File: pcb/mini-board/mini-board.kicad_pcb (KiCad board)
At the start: 4 copper layers, 132.1 x 132.1 mm, 55 parts, among them J1 USB_B, J2 EXPANSION BUS, J3 SD Card Board, J4 Atmel-JTAG-10, J5 SYSTEM BUS, J8 SERIAL, SW1 SW_SPDT, SW2 RESET, SW3 NMI, U1 74AC11, U11 DS1813, U15 SST39SF040, U16 AS6C4008-55, U19 W65C22S, U2 W65C02, U21 W65C51N, U22 MAX232, U23 ATF1502AS, X1 CLK, Y1 1.8432 MHz

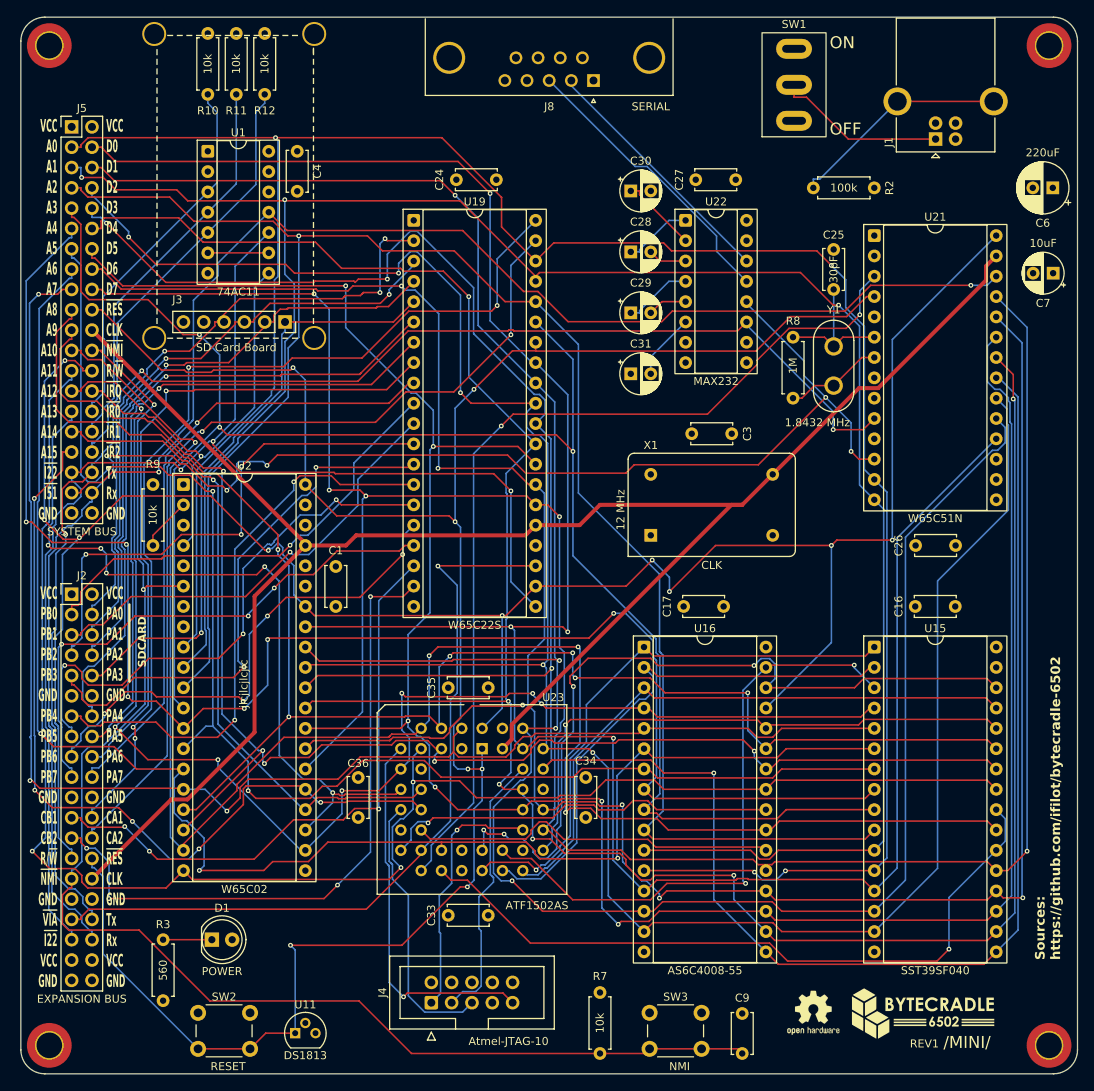
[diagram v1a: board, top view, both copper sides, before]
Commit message: Rivising board
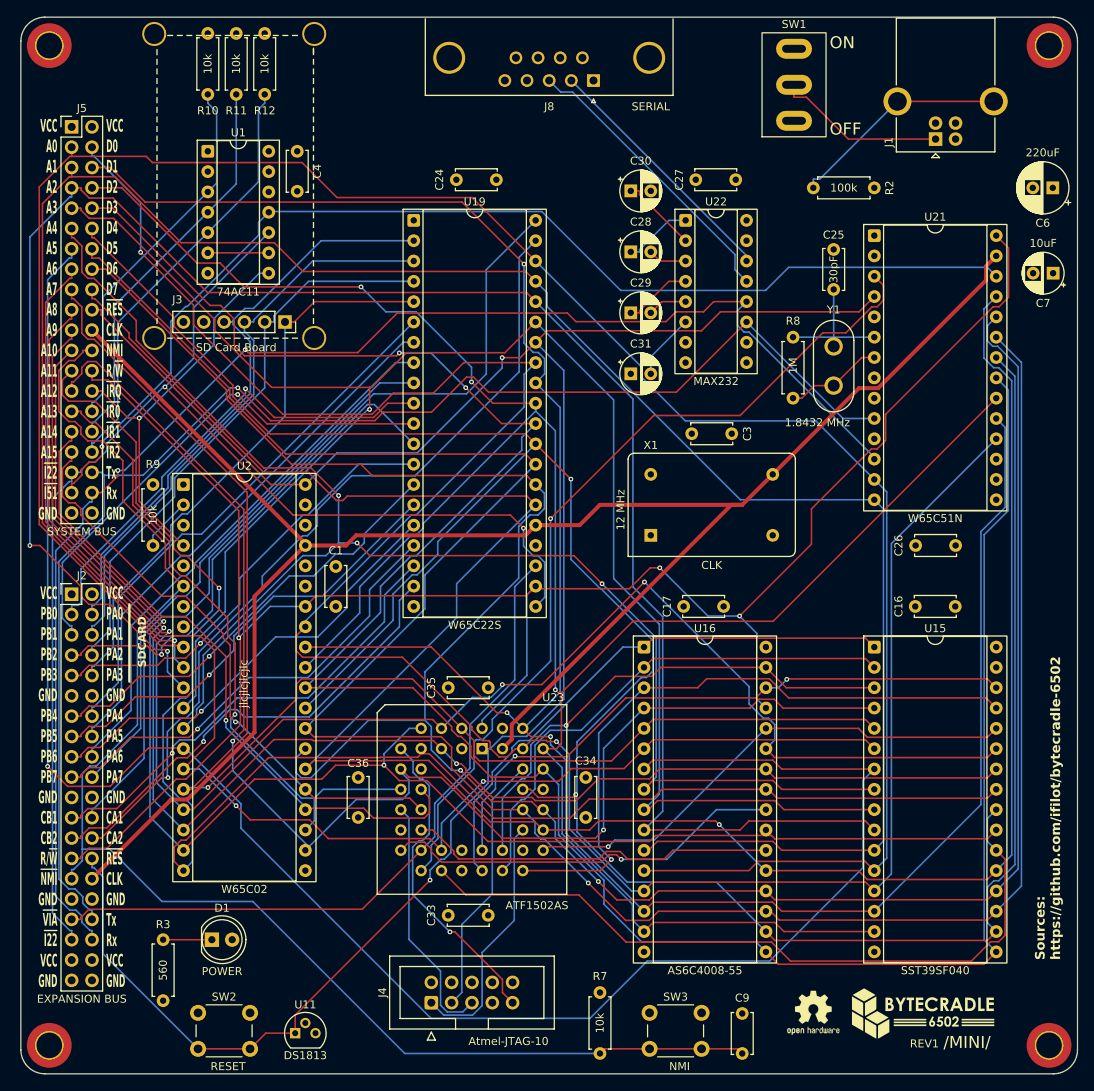
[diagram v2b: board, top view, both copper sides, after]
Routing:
- net A5: track 174.8 -> 237.3 mm, vias 3 -> 1
- net GND: track 30.0 -> 65.5 mm
- net VCC: track 31.3 -> 65.3 mm
- net R/~{W}: track 277.3 -> 246.6 mm, vias 9 -> 3
- net A15: track 103.1 -> 73.3 mm, vias 5 -> 1
- net A10: track 216.7 -> 190.5 mm, vias 4 -> 2
- net CB2: track 83.8 -> 59.0 mm, vias 4 -> 1
- net A6: track 195.8 -> 176.0 mm, vias 3 -> 2
- net B4: track 97.3 -> 78.2 mm, vias 4 -> 2
- net D4: track 294.8 -> 313.8 mm, vias 6 -> 2
- net CB1: track 75.6 -> 58.3 mm, vias 3 -> 1
- net A13: track 96.5 -> 79.5 mm, vias 5 -> 1
- net PB4: track 71.5 -> 55.6 mm, vias 2 -> 1
- net PA6: track 83.7 -> 67.8 mm, vias 1 -> 0
- net PA4: track 82.8 -> 67.5 mm, vias 1 -> 0
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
